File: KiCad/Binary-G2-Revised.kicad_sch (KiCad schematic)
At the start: 91 parts, among them J1 USB_C_Receptacle_PowerOnly_6P, J2 Conn_01x01, J3 Conn_01x01, SW1 PTH_RA_7.4x4.3mm, SW2 PTH_RA_7.4x4.3mm, SW3 PTH_RA_7.4x4.3mm, SW4 SW_SPDT, U1 74HC4060, U10 BQ21040DBV, U12 MCP65R41-2402, U13 MCP65R41-2402, U2 74HC14, U3 74LS32, U4 74LS08, U5 74LS08, U6 74LS393, U7 74LS393, U8 74LS393, U9 74LS393, Y1 32.768Khz

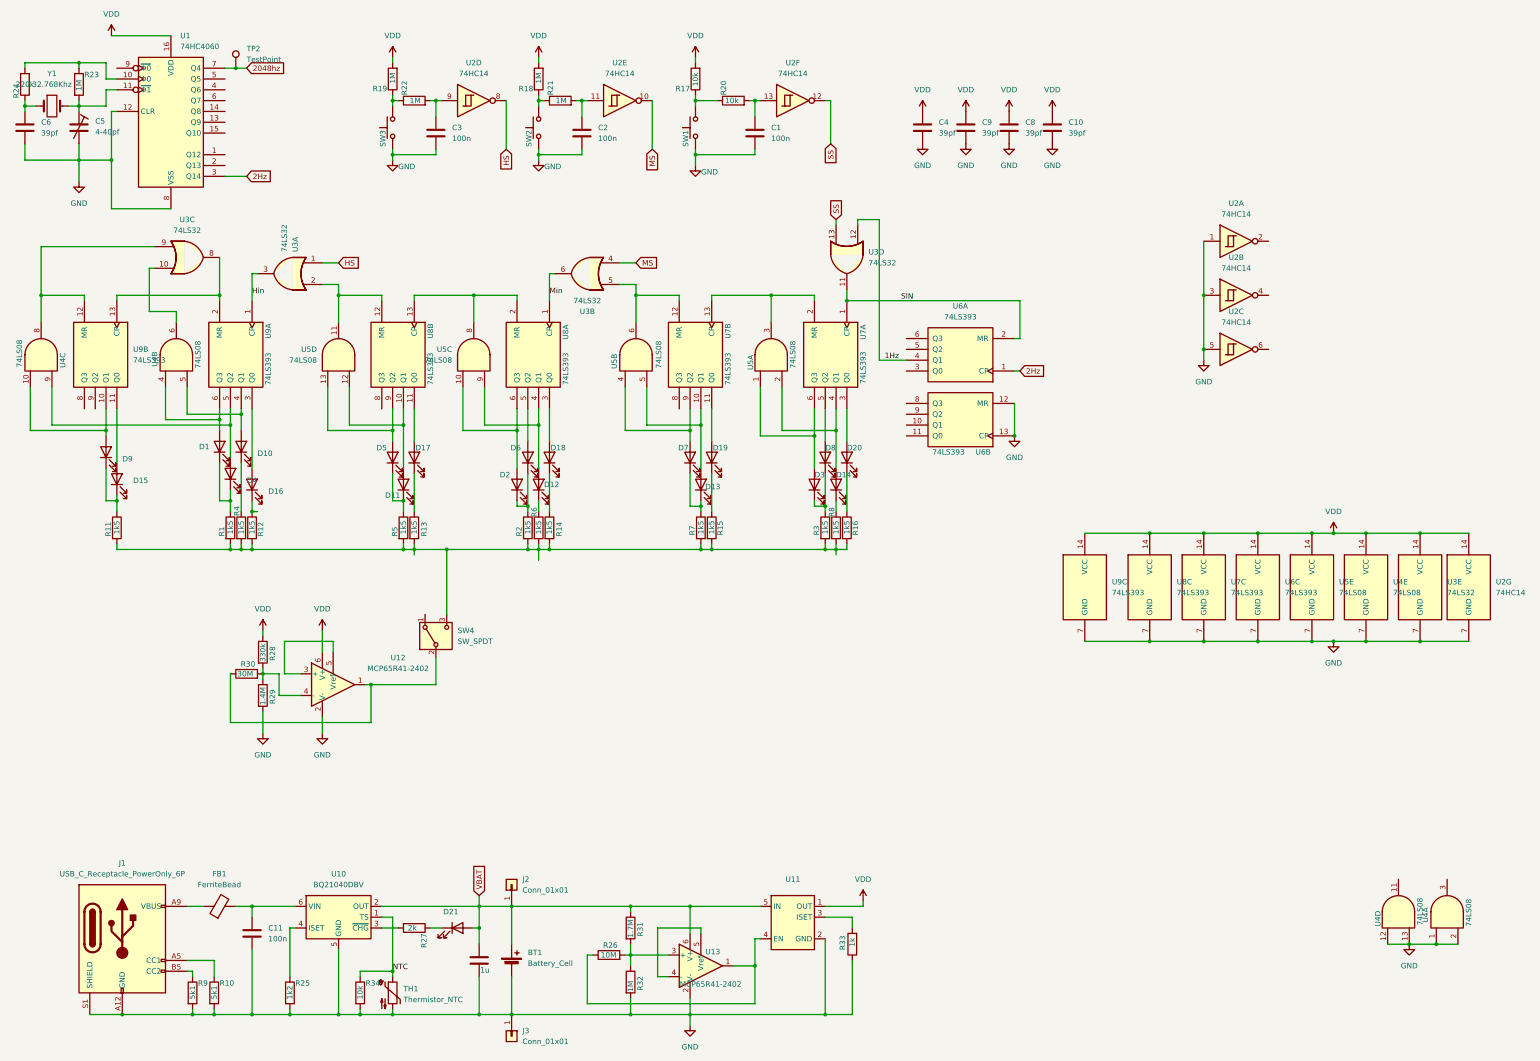
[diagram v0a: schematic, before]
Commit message: Quick Update Documentation
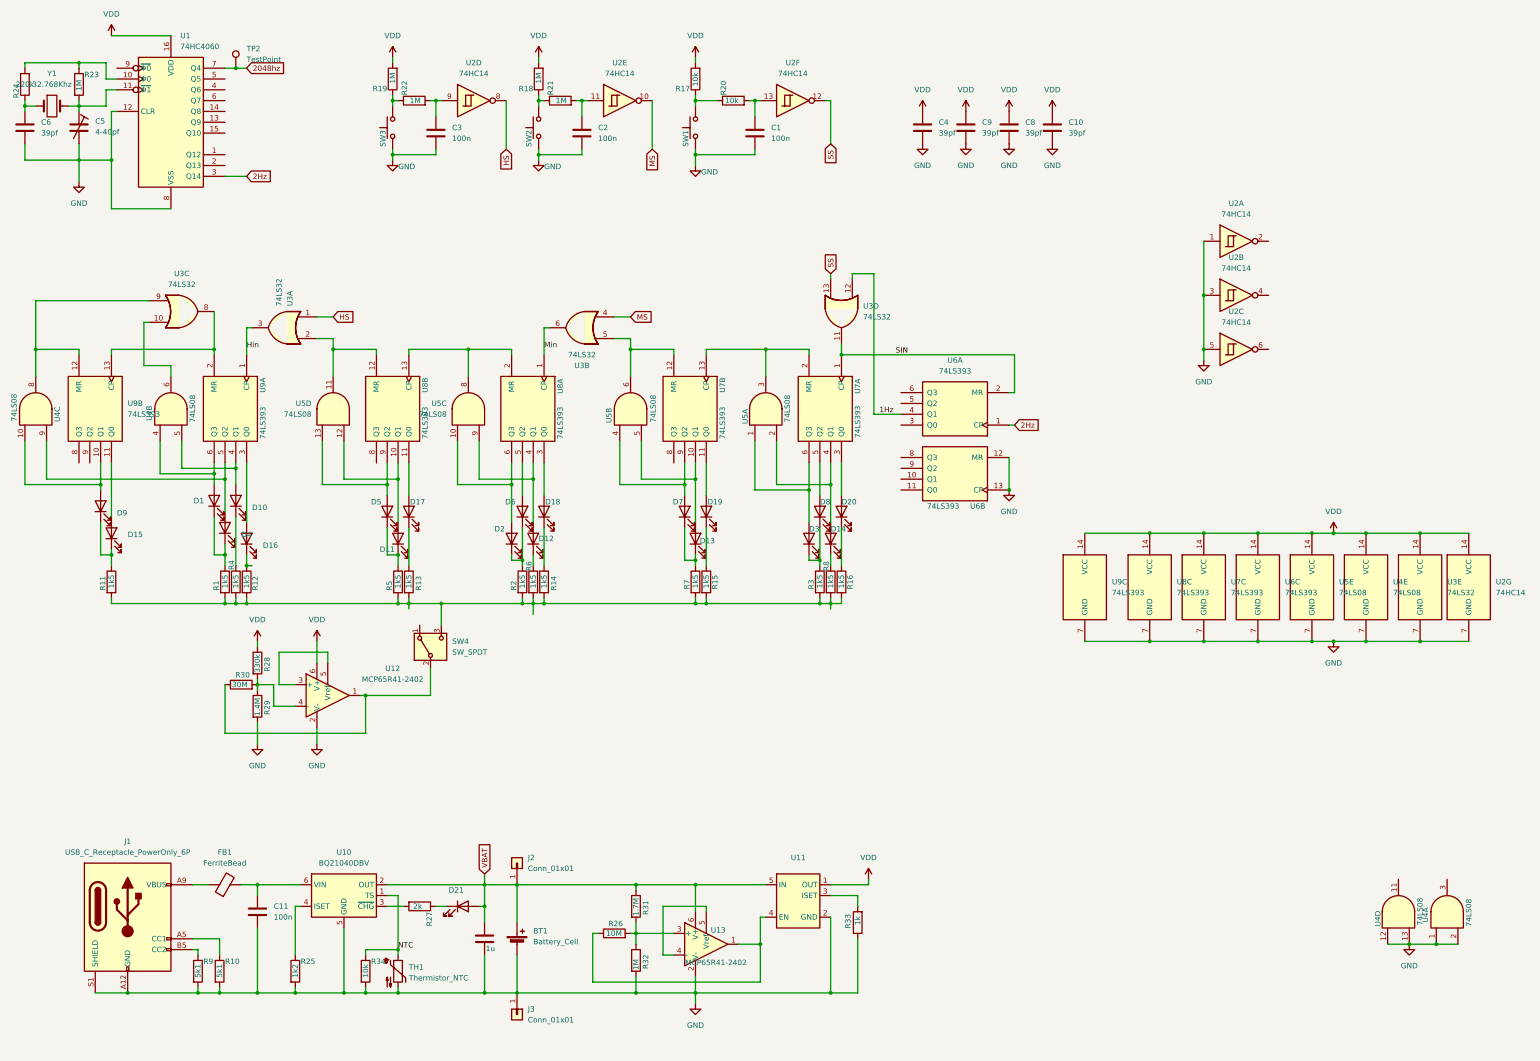
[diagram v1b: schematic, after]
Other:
- moved on the sheet: BT1, C11, D1, D10, D11, D12, D13, D14, D15, D16, D17, D18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
